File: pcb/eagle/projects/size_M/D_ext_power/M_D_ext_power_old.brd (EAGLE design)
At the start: 20 parts

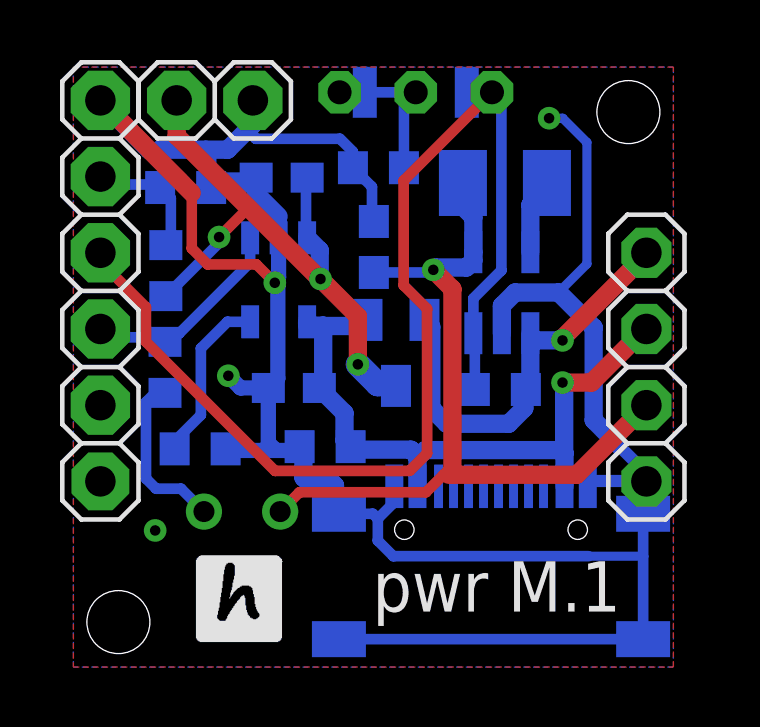
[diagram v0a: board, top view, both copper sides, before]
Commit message: PCB M.1
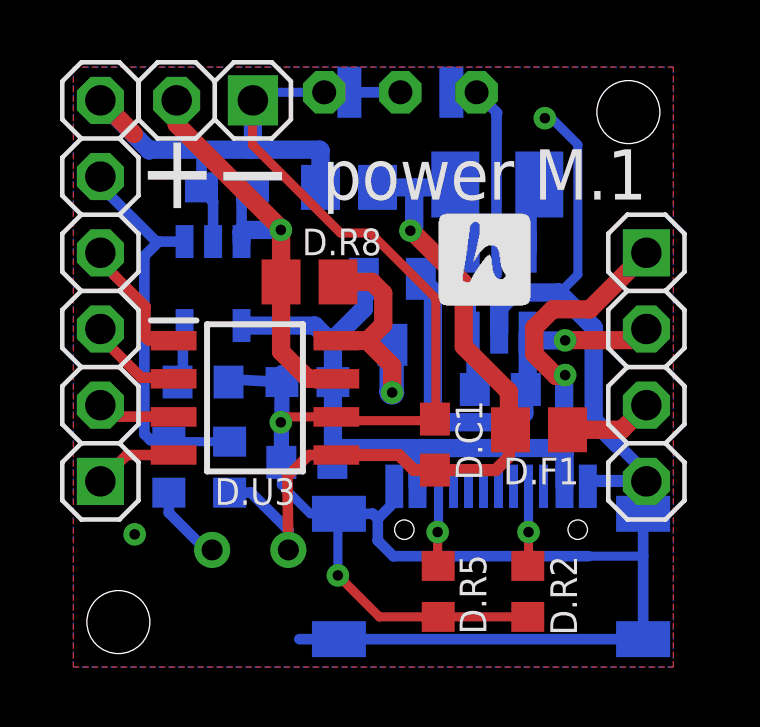
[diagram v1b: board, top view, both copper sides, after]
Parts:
- added D.C1: 100n, rcl:C0603
- added D.F1: (no value), rcl:R0805
- added D.R8: 0.1, rcl:R0805
- added D.U3: INA219AIDR, SamacSys_Parts:SOIC127P600X175-8N
- D.C7: value 10u -> 22u; device rcl:C0603 -> rcl:C0805
- D.R1: value 3k3 -> 100k
- D.R2, D.R5: value 100k -> 5k1
- D.R3: value 22k -> 12k
- D.R6: value 150 -> 2k2
- D.U2: value TC -> LM3671_3.3
- moved D.R2 16.1 mm to (15.6, 3.02), flipped to the top
- moved D.R5 15.9 mm to (12.7, 3.02), flipped to the top, turned to 270 degrees
- moved D.R1 11.1 mm to (5.71, 7.17), turned to 90 degrees
- moved D.R6 3.33 mm to (3.68, 7.16)
- moved D.R3 2.23 mm to (4.82, 10.0)
- moved D.U1 2.19 mm to (5.16, 13.2)
- moved D.C7 2.15 mm to (9.69, 16.5), turned to 180 degrees
- moved D.C6 1.85 mm to (5.62, 16.5)
- moved D.T1 1.37 mm to (11.1, 12.3)
- moved D.D1 1.31 mm to (6.40, 4.01)
- moved D.R4 0.80 mm to (8.28, 7.32)
- moved D.ON/OFF/RESET 0.51 mm to (11.4, 19.7)
- moved D.C4 0.49 mm to (8.30, 10.0)
- moved D.L1 0.26 mm to (14.6, 16.6)
- moved D.U2 0.09 mm to (14.7, 13.0)
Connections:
- removed net N$20: D.J2.4, D.ON/OFF/RESET.P$1, D.ON/OFF/RESET.P$4, D.R7.2, D.U2.SHDN
- removed net PA7: D.J2.3, D.R6.1, D.U1.1
- new net N$13: D.C6.2, D.LIPOL.2, D.R8.2, D.U1.3, D.U3.7
- new net N$4: D.R5.1, U$1.B5
- new net N$6: D.R2.1, U$1.A5
- new net P0: D.J2.4, D.U3.1
- new net P1: D.J2.3, D.U3.2
- new net P4: D.J2.5, D.R1.2, D.R6.1, D.U1.1
- new net SCL: D.J2.1, D.U3.4
- new net SDA: D.J2.2, D.U3.3
- net GND: now also D.C1.1, D.ON/OFF/RESET.P$2, D.ON/OFF/RESET.P$3, D.ON/OFF/RESET.P$5, D.R2.2, D.R5.2, D.U3.6; no longer D.R1.2, D.R5.1
- net N$1: now also D.F1.2, D.J3.3; no longer D.ON/OFF/RESET.P$2, D.ON/OFF/RESET.P$3, D.ON/OFF/RESET.P$5, D.R1.1
- net N$12: now also D.J3.2; no longer D.J3.1
- net N$5: now also D.ON/OFF/RESET.P$1, D.ON/OFF/RESET.P$4, D.R7.2, D.U2.SHDN; no longer D.J2.5, D.R2.1, D.R5.2
- net N$8: now also D.R8.1, D.U3.8; no longer D.C6.2, D.LIPOL.2, D.R2.2, D.U1.3
- net N$9: now also D.J3.1; no longer D.J3.2
- net VDD: now also D.C1.2, D.F1.1, D.R1.1, D.U3.5; no longer D.J3.3
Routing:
- net N$20: track 39.9 -> 0.00 mm
- net GND: track 92.0 -> 108.5 mm
- net N$13: track 0.00 -> 16.0 mm, vias 0 -> 1
- net P4: track 0.00 -> 14.6 mm
- net N$8: track 20.6 -> 9.31 mm, vias 3 -> 1
- net N$9: track 23.3 -> 33.0 mm
- net PA7: track 7.50 -> 0.00 mm
- net N$5: track 4.29 -> 11.4 mm
- net P0: track 0.00 -> 4.43 mm
- net VDD: track 27.7 -> 31.5 mm
- net P1: track 0.00 -> 3.62 mm
- net N$11: track 5.72 -> 2.19 mm
- net SCL: track 0.00 -> 2.81 mm
- net N$3: track 6.06 -> 3.32 mm
- net N$6: track 0.00 -> 2.66 mm, vias 0 -> 1
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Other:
- board text added: "+"
- board text added: "power M.1"
- board text added: "−"
- board text removed: "pwr M.1"
